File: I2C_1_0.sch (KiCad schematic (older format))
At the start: 2 parts, among them U1 PCA9306

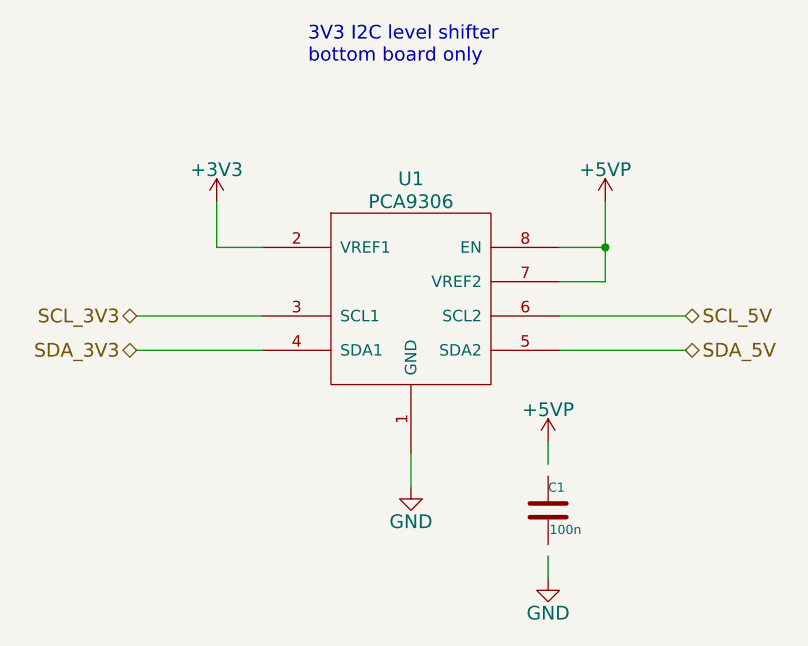
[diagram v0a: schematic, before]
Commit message: Final production board v1.0
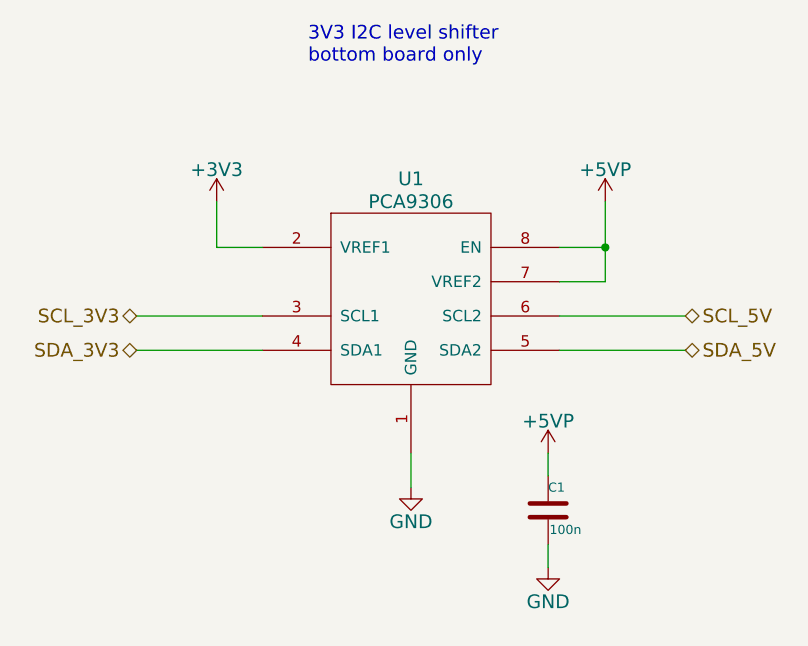
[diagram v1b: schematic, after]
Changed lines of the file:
@@
 EESchema Schematic File Version 2
+LIBS:MicroFLiC_servo_solenoid_1_0-rescue
 LIBS:power
 LIBS:device
@@
 L GND #PWR013
 U 1 1 54D9606F
-P 5450 3950
-F 0 "#PWR013" H 5450 3700 60  0001 C CNN
-F 1 "GND" H 5450 3800 60  0000 C CNN
-F 2 "" H 5450 3950 60  0000 C CNN
-F 3 "" H 5450 3950 60  0000 C CNN
-	1    5450 3950
+P 5450 3900
+F 0 "#PWR013" H 5450 3650 60  0001 C CNN
+F 1 "GND" H 5450 3750 60  0000 C CNN
+F 2 "" H 5450 3900 60  0000 C CNN
+F 3 "" H 5450 3900 60  0000 C CNN
+	1    5450 3900
 	1    0    0    -1
 $EndComp
@@
 U 1 1 54D96092
 P 5450 3650
+AR Path="/54D96092" Ref="C1"  Part="1"
+AR Path="/54D957C7/54D96092" Ref="C1"  Part="1"
 F 0 "C1" H 5450 3750 40  0000 L CNN
 F 1 "100n" H 5456 3565 40  0000 L CNN
@@
 $EndComp
 Wire Wire Line
-	5450 3450 5450 3350
+	5450 3500 5450 3400
 Wire Wire Line
-	5450 3950 5450 3850
+	5450 3900 5450 3800
 $Comp
 L +5VP #PWR014
 U 1 1 54D960F9
-P 5450 3350
-F 0 "#PWR014" H 5450 3200 60  0001 C CNN
-F 1 "+5VP" H 5450 3490 60  0000 C CNN
-F 2 "" H 5450 3350 60  0000 C CNN
-F 3 "" H 5450 3350 60  0000 C CNN
-	1    5450 3350
+P 5450 3400
+F 0 "#PWR014" H 5450 3250 60  0001 C CNN
+F 1 "+5VP" H 5450 3540 60  0000 C CNN
+F 2 "" H 5450 3400 60  0000 C CNN
+F 3 "" H 5450 3400 60  0000 C CNN
+	1    5450 3400
 	1    0    0    -1
 $EndComp
